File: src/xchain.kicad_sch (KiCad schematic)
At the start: 11 parts, among them Q1 PNP, Q2 PNP, SW1 SW_Push, SW2 SW_Push

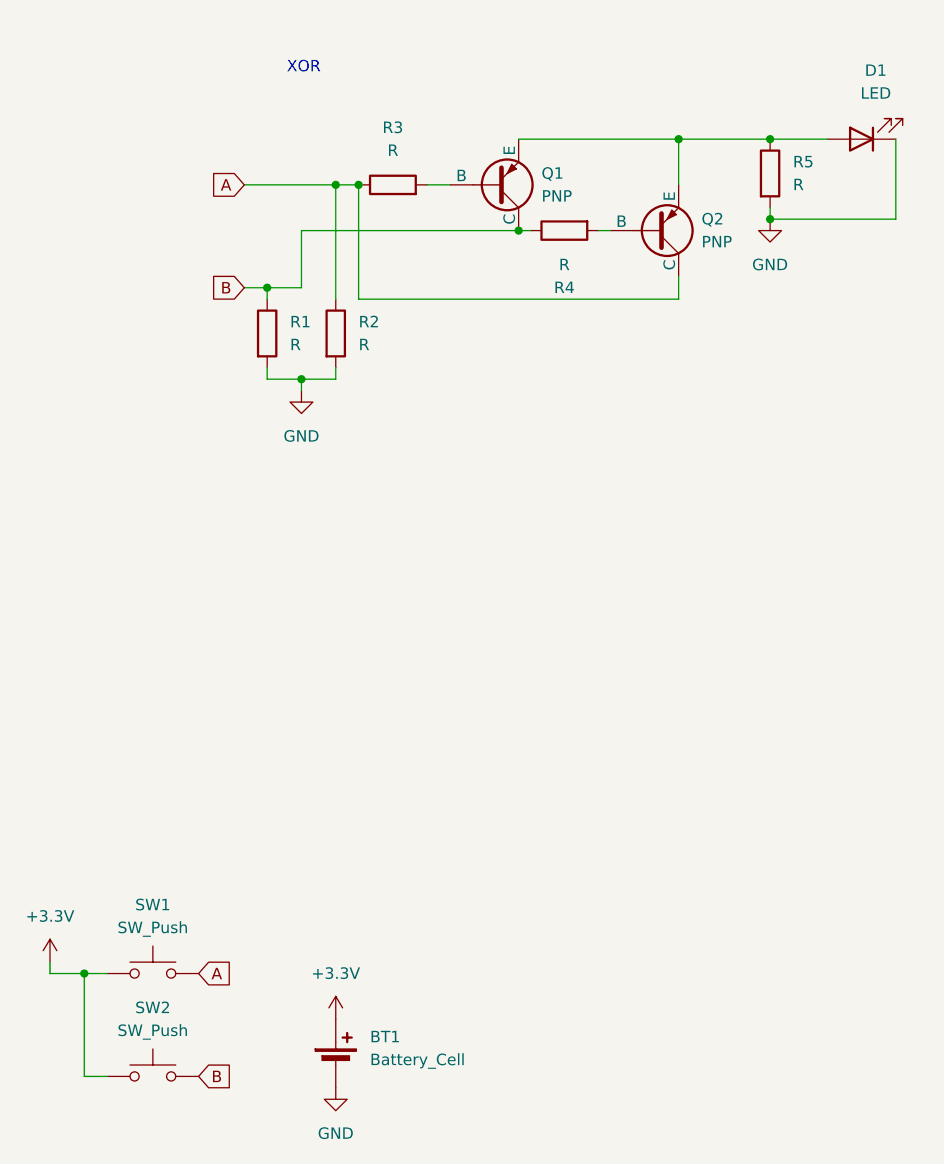
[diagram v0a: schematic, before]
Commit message: Revision
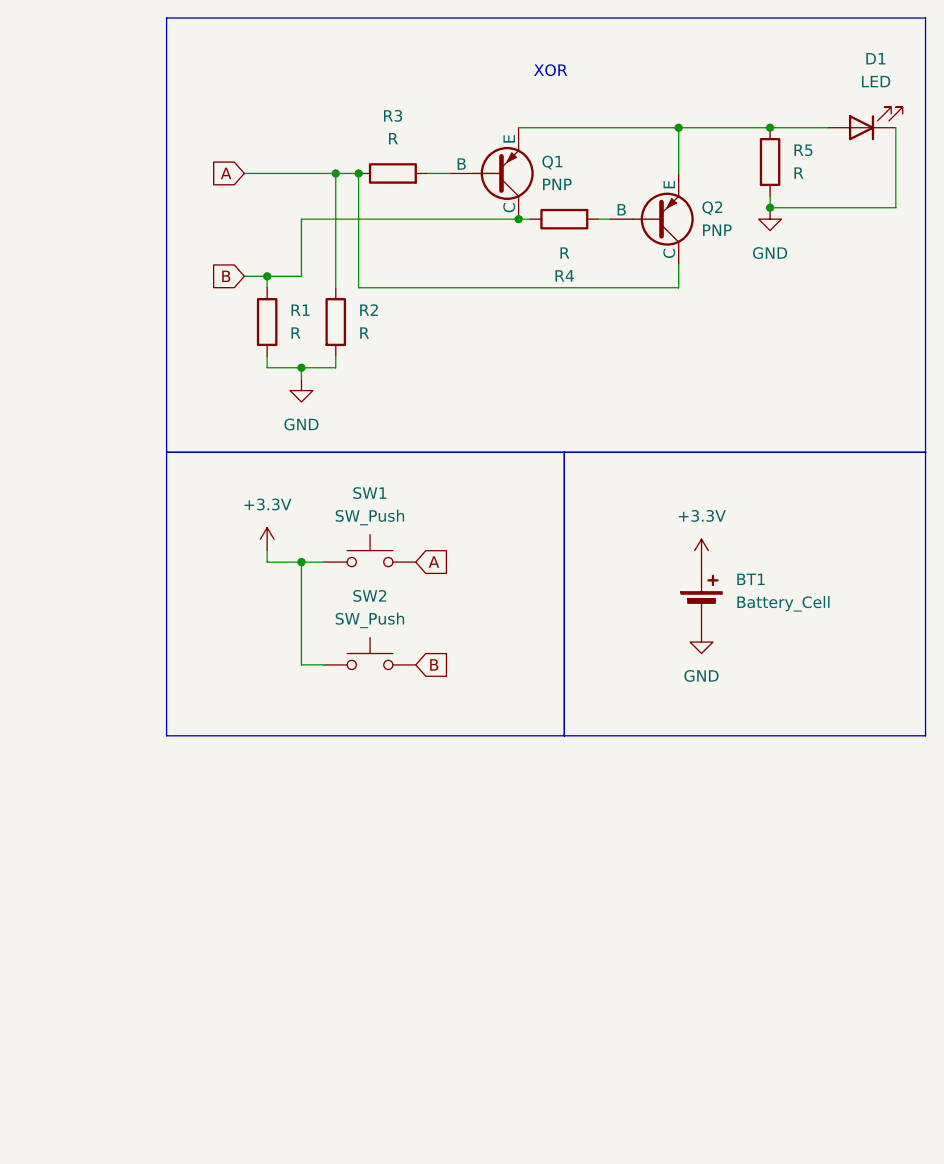
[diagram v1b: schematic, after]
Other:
- moved on the sheet: BT1, D1, Q1, Q2, R1, R2, R3, R4, R5, SW1, SW2
